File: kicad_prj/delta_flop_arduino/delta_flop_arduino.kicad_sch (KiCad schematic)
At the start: 1 part, among them U1 Arduino_Nano

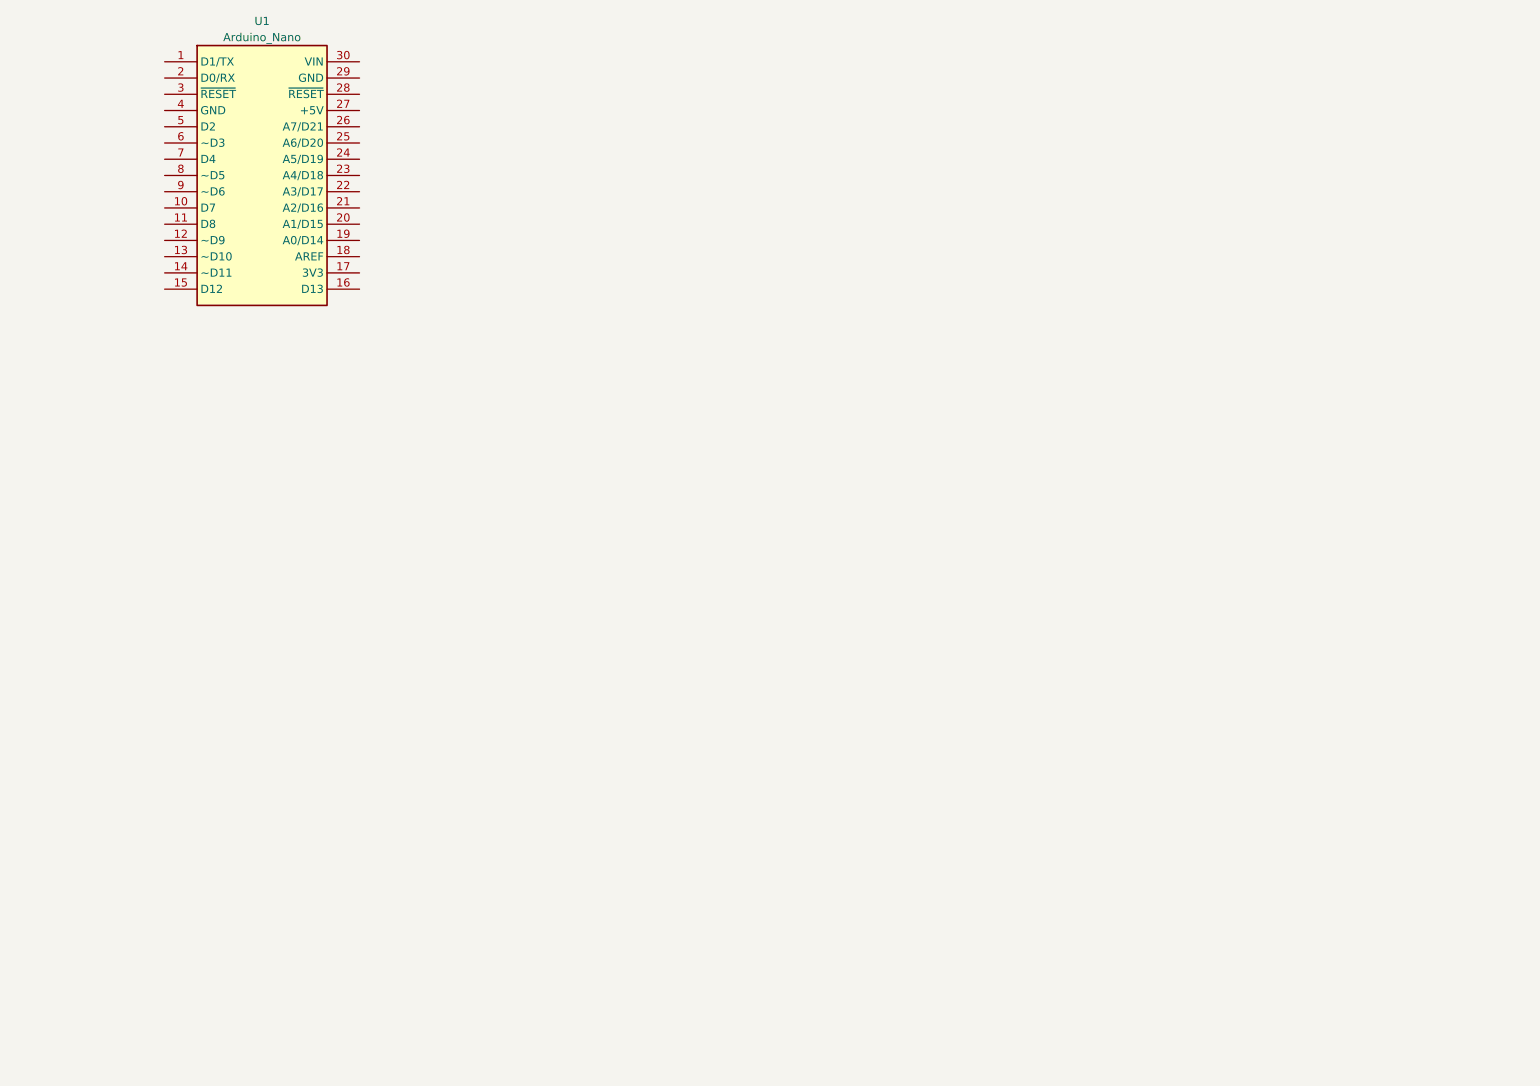
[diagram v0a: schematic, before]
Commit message: Pre-version made
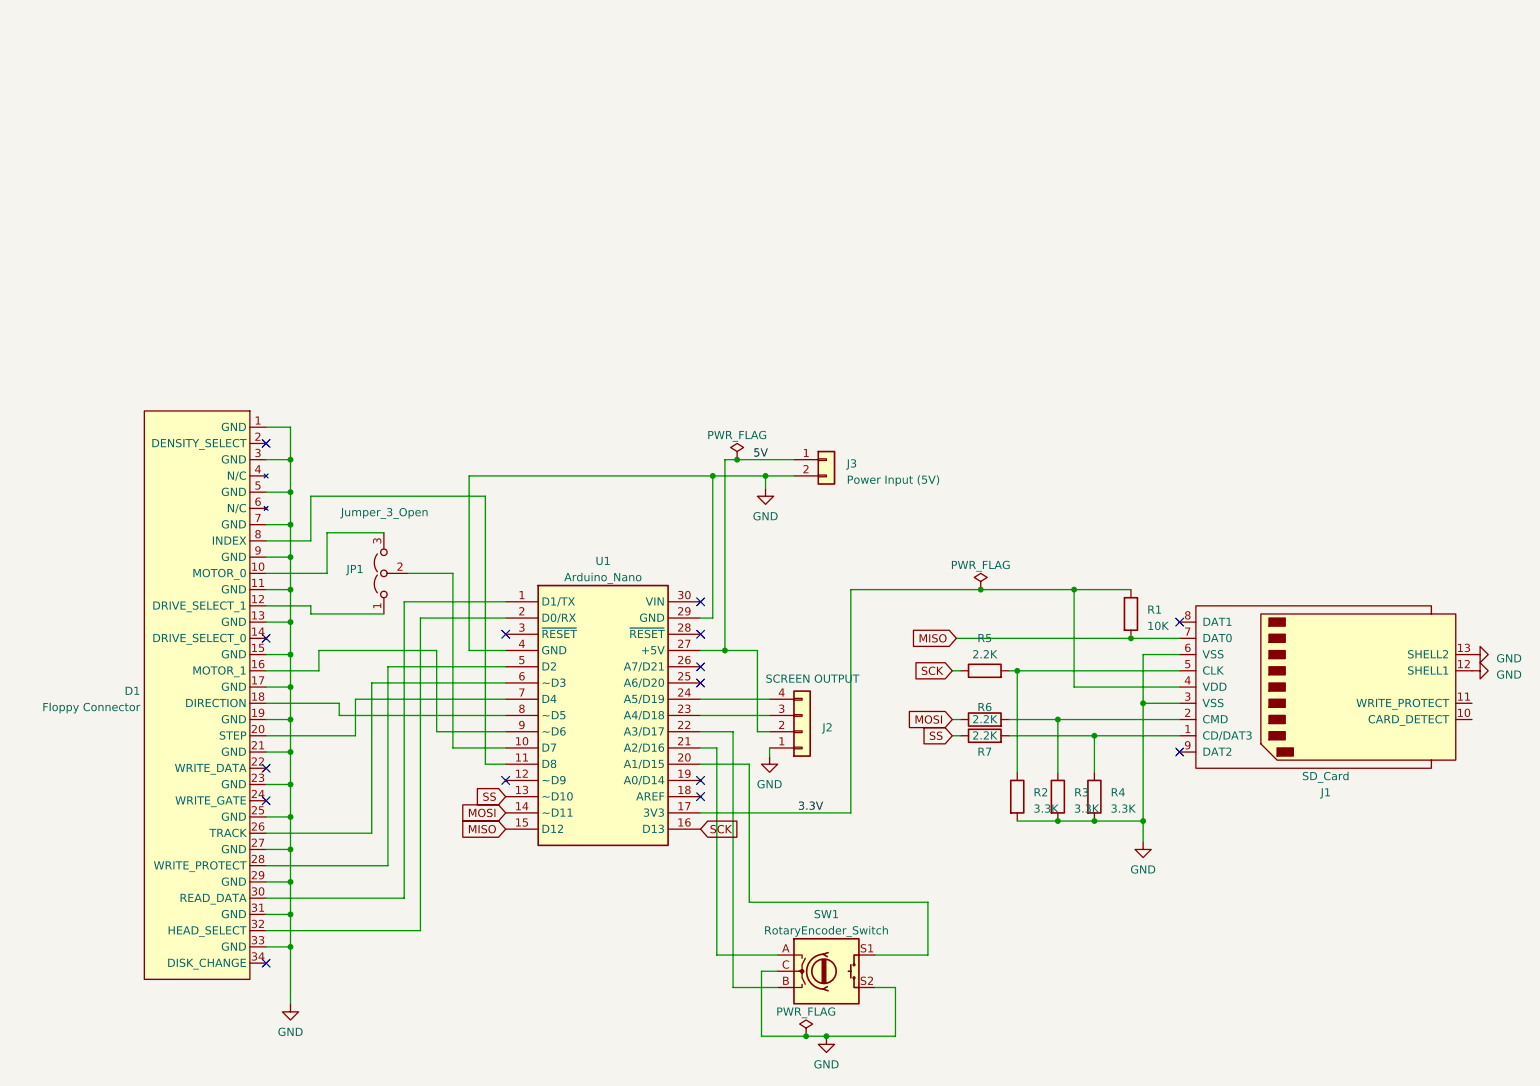
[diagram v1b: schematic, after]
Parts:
- added D1: Floppy Connector, Connector_IDC:IDC-Header_2x17_P2.54mm_Vertical, symbol delta_flop_pre:34_pin_floppy_convertor
- added J1: SD_Card, delta_flop_pre:SDCARD_4UCONN, symbol delta_flop_pre:SD_Card
- added J2: SCREEN OUTPUT, Connector_PinHeader_2.54mm:PinHeader_1x04_P2.54mm_Vertical, symbol delta_flop_pre:Conn_01x04
- added J3: Power Input (5V), Connector_PinHeader_2.54mm:PinHeader_1x02_P2.54mm_Vertical, symbol Connector_Generic:Conn_01x02
- added JP1: Jumper_3_Open, Connector_PinHeader_2.54mm:PinHeader_1x03_P2.54mm_Vertical, symbol Jumper:Jumper_3_Open
- added R1: 10K, R_Axial_DIN0207_L6.3mm_D2.5mm_P10.16mm_Horizontal, symbol Device:R
- added R2, R3, R4: 3.3K, R_Axial_DIN0207_L6.3mm_D2.5mm_P10.16mm_Horizontal, symbol Device:R
- added R5, R6, R7: 2.2K, R_Axial_DIN0207_L6.3mm_D2.5mm_P10.16mm_Horizontal, symbol Device:R
- added SW1: RotaryEncoder_Switch, Rotary_Encoder:RotaryEncoder_Alps_EC11E-Switch_Vertical_H20mm, symbol delta_flop_pre:RotaryEncoder_Switch
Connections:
- net at U1.1 (D1/TX): now also D1.30 (READ_DATA)
- net at U1.10 (D7): now also JP1.2 (C)
- net at U1.11 (D8): now also D1.8 (INDEX)
- net SS: now reaches U1.13 (~D10)
- net SS: now also R7.1
- net MOSI: now reaches U1.14 (~D11)
- net MOSI: now also R6.1
- net MISO: now reaches U1.15 (D12)
- net MISO: now also J1.7 (DAT0), R1.2
- net SCK: now reaches U1.16 (D13)
- net SCK: now also R5.1
- net 3.3V: now reaches U1.17 (3V3)
- net 3.3V: now also J1.4 (VDD), R1.1
- net at U1.2 (D0/RX): now also D1.32 (HEAD_SELECT)
- net at U1.20 (A1/D15): now also SW1.S1
- net at U1.21 (A2/D16): now also SW1.A
- net at U1.22 (A3/D17): now also SW1.B
- net at U1.23 (A4/D18): now also J2.3 (Pin_3)
- net at U1.24 (A5/D19): now also J2.4 (Pin_4)
- net 5V: now reaches U1.27 (+5V)
- net 5V: now also J2.2 (Pin_2), J3.1 (Pin_1)
- net GND: now reaches U1.29 (GND)
- net GND: now also U1.4 (GND), D1.1 (GND), D1.11 (GND), D1.13 (GND), D1.15 (GND), D1.17 (GND), D1.19 (GND), D1.21 (GND), D1.23 (GND), D1.25 (GND), D1.27 (GND), D1.29 (GND), D1.3 (GND), D1.31 (GND), D1.33 (GND), D1.5 (GND), D1.7 (GND), D1.9 (GND), J1.12 (SHELL1), J1.13 (SHELL2), J1.3 (VSS), J1.6 (VSS), J2.1 (Pin_1), J3.2 (Pin_2), R2.2, R3.2, R4.2, SW1.C, SW1.S2
- net at U1.5 (D2): now also D1.28 (WRITE_PROTECT)
- net at U1.6 (~D3): now also D1.26 (TRACK)
- net at U1.7 (D4): now also D1.20 (STEP)
- net at U1.8 (~D5): now also D1.18 (DIRECTION)
- net at U1.9 (~D6): now also D1.16 (MOTOR_1)
- new net: J1.5 (CLK), R2.1, R5.2
- new net: J1.2 (CMD), R3.1, R6.2
- new net: D1.12 (DRIVE_SELECT_1), JP1.1 (A)
- new net: D1.10 (MOTOR_0), JP1.3 (B)
- new net: J1.1 (CD/DAT3), R4.1, R7.2
- no-connect marks 0 -> 15
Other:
- moved on the sheet: U1
